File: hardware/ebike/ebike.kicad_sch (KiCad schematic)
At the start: 19 parts, among them U1 STM32G431CBTx, Y1 ABLS-8MHZ-B2-T

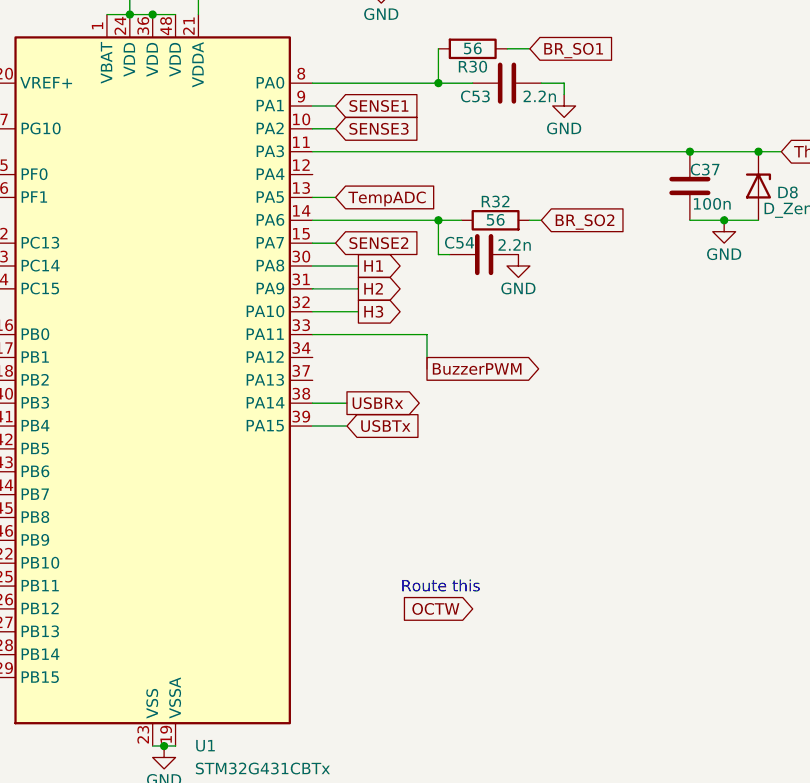
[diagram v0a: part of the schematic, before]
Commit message: finished annoation for schematic
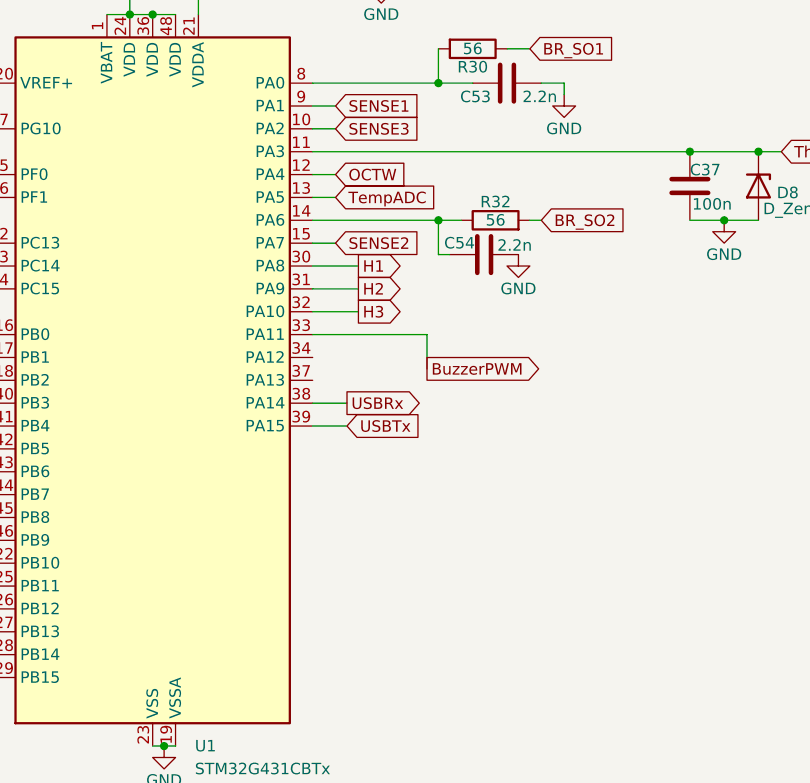
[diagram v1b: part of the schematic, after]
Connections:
- net OCTW: now also U1.12 (PA4)
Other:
- note removed: "Route this"
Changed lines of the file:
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@@
-		)
-	)
-	(text "Route this\n"
-		(exclude_from_sim no)
-		(at 183.134 114.554 0)
-		(effects
-			(font
-				(size 1.27 1.27)
-			)
 		)
 	)
@@
 		(pts
 			(xy 184.15 77.47) (xy 182.88 77.47)
+		)
+		(stroke
+			(width 0)
+			(type default)
+		)
+	)
+	(wire
+		(pts
+			(xy 168.91 68.58) (xy 171.45 68.58)
 		)
 		(stroke
@@
 	(global_label "OCTW"
 		(shape input)
-		(at 186.69 116.84 180)
+		(at 171.45 68.58 0)
 		(fields_autoplaced yes)
 		(effects
@@
 				(size 1.27 1.27)
 			)
-			(justify right)
+			(justify left)
 		)
 		(property "Intersheetrefs" "${INTERSHEET_REFS}"
-			(at 178.6853 116.84 0)
+			(at 179.4547 68.58 0)
 			(effects
 				(font
 					(size 1.27 1.27)
 				)
-				(justify right)
+				(justify left)
 				(hide yes)
 			)
